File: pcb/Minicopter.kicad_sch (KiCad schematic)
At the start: 0 parts

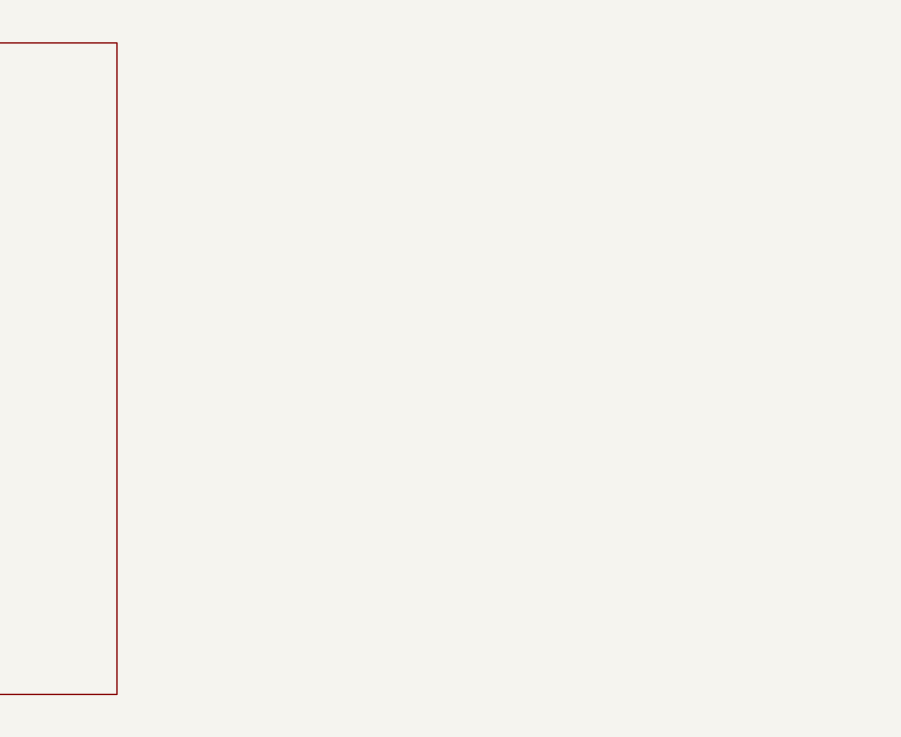
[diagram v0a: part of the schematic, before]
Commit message: battery
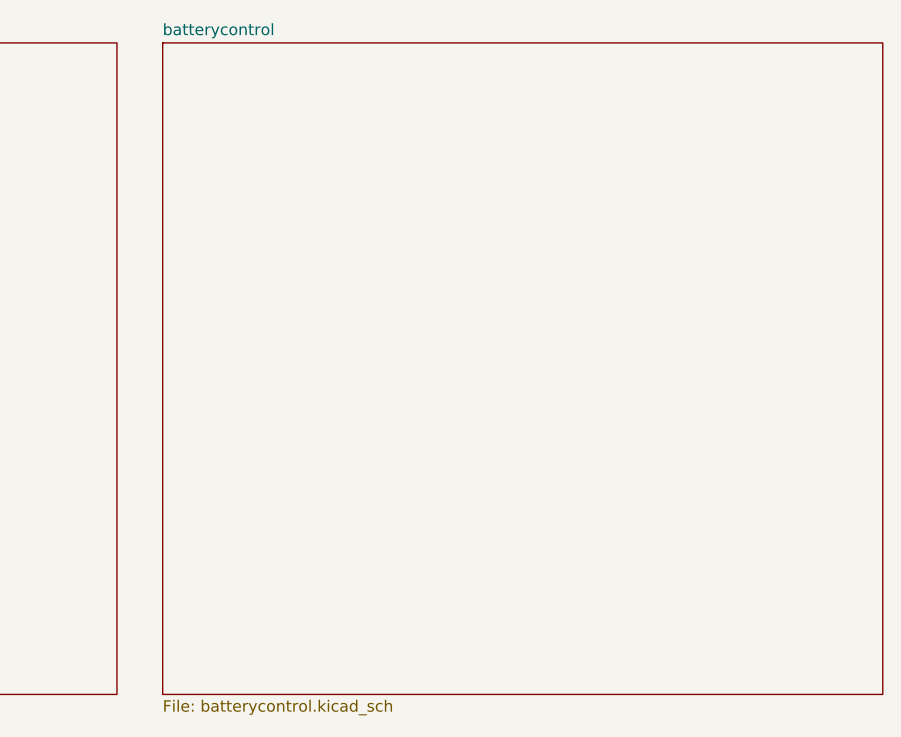
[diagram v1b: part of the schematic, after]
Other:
- added sheet batterycontrol (batterycontrol.kicad_sch)
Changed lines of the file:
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@@
+	)
+	(sheet
+		(at 201.93 17.78)
+		(size 80.01 72.39)
+		(exclude_from_sim no)
+		(in_bom yes)
+		(on_board yes)
+		(dnp no)
+		(fields_autoplaced yes)
+		(stroke
+			(width 0.1524)
+			(type solid)
+		)
+		(fill
+			(color 0 0 0 0.0000)
+		)
+		(property "Sheetname" "batterycontrol"
+			(at 201.93 17.0684 0)
+			(effects
+				(font
+					(size 1.27 1.27)
+				)
+				(justify left bottom)
+			)
+		)
+		(property "Sheetfile" "batterycontrol.kicad_sch"
+			(at 201.93 90.7546 0)
+			(effects
+				(font
+					(size 1.27 1.27)
+				)
+				(justify left top)
+			)
+		)
+		(instances
+			(project "Minicopter"
+				(path "/64f47f0f-737f-4ea8-9b68-9c8ed6450afb"
+					(page "4")
+				)
+			)
+		)
 	)
 	(sheet

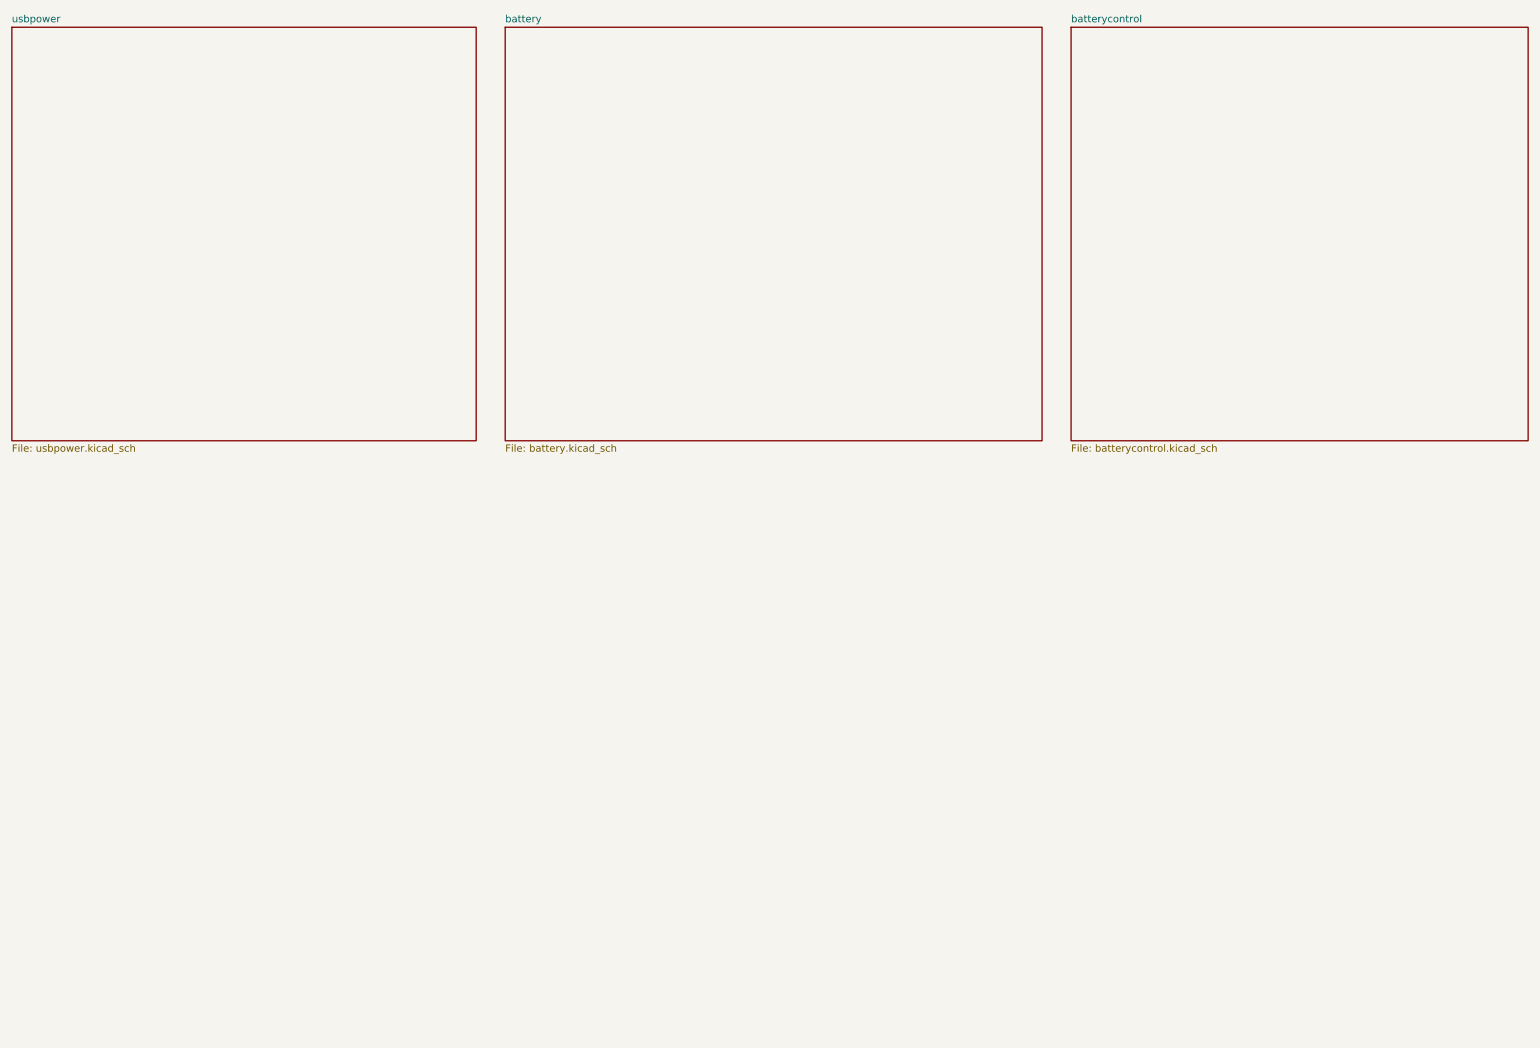
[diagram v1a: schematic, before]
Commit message: with errors
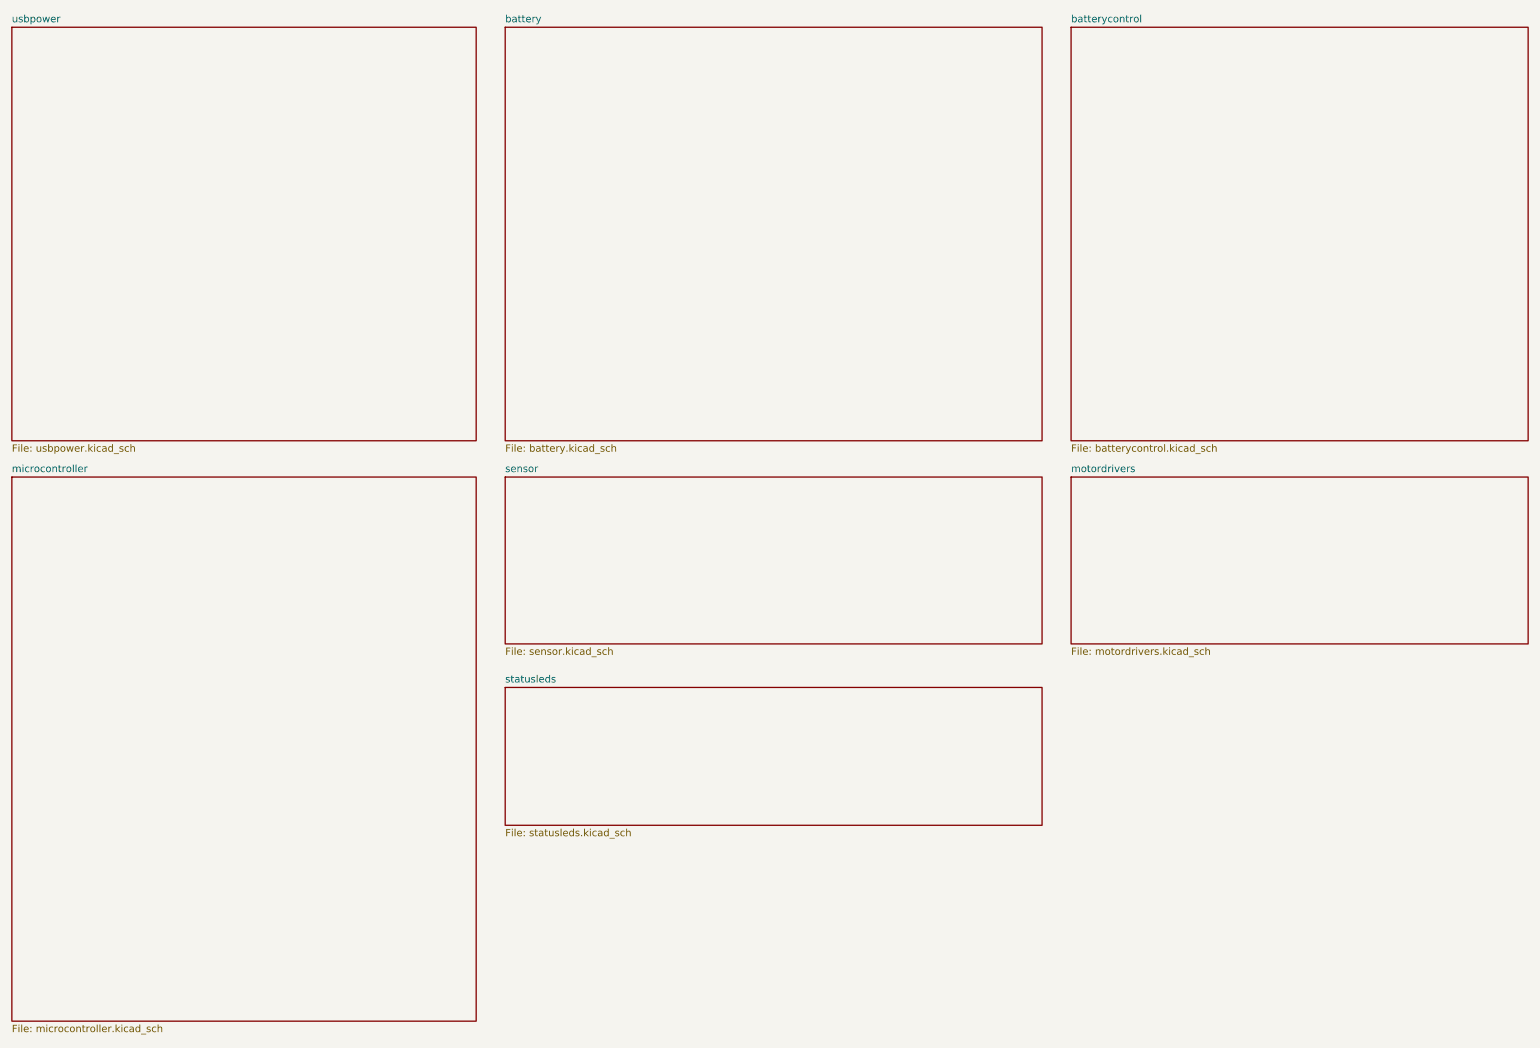
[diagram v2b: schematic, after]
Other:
- added sheet microcontroller (microcontroller.kicad_sch)
- added sheet motordrivers (motordrivers.kicad_sch)
- added sheet sensor (sensor.kicad_sch)
- added sheet statusleds (statusleds.kicad_sch)
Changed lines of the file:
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@@
+	)
+	(sheet
+		(at 16.51 96.52)
+		(size 81.28 95.25)
+		(exclude_from_sim no)
+		(in_bom yes)
+		(on_board yes)
+		(dnp no)
+		(fields_autoplaced yes)
+		(stroke
+			(width 0.1524)
+			(type solid)
+		)
+		(fill
+			(color 0 0 0 0.0000)
+		)
+		(property "Sheetname" "microcontroller"
+			(at 16.51 95.8084 0)
+			(effects
+				(font
+					(size 1.27 1.27)
+				)
+				(justify left bottom)
+			)
+		)
+		(property "Sheetfile" "microcontroller.kicad_sch"
+			(at 16.51 192.3546 0)
+			(effects
+				(font
+					(size 1.27 1.27)
+				)
+				(justify left top)
+			)
+		)
+		(instances
+			(project "Minicopter"
+				(path "/64f47f0f-737f-4ea8-9b68-9c8ed6450afb"
+					(page "5")
+				)
+			)
+		)
 	)
 	(sheet
@@
 				)
 			)
+		)
+	)
+	(sheet
+		(at 102.87 96.52)
+		(size 93.98 29.21)
+		(exclude_from_sim no)
+		(in_bom yes)
+		(on_board yes)
+		(dnp no)
+		(fields_autoplaced yes)
+		(stroke
+			(width 0.1524)
+			(type solid)
+		)
+		(fill
+			(color 0 0 0 0.0000)
+		)
+		(property "Sheetname" "sensor"
+			(at 102.87 95.8084 0)
+			(effects
+				(font
+					(size 1.27 1.27)
+				)
+				(justify left bottom)
+			)
+		)
+		(property "Sheetfile" "sensor.kicad_sch"
+			(at 102.87 126.3146 0)
+			(effects
+				(font
+					(size 1.27 1.27)
+				)
+				(justify left top)
+			)
+		)
+		(instances
+			(project "Minicopter"
+				(path "/64f47f0f-737f-4ea8-9b68-9c8ed6450afb"
+					(page "6")
+				)
+			)
+		)
+	)
+	(sheet
+		(at 201.93 96.52)
+		(size 80.01 29.21)
+		(exclude_from_sim no)
+		(in_bom yes)
+		(on_board yes)
+		(dnp no)
+		(fields_autoplaced yes)
+		(stroke
+			(width 0.1524)
+			(type solid)
+		)
+		(fill
+			(color 0 0 0 0.0000)
+		)
+		(property "Sheetname" "motordrivers"
+			(at 201.93 95.8084 0)
+			(effects
+				(font
+					(size 1.27 1.27)
+				)
+				(justify left bottom)
+			)
+		)
+		(property "Sheetfile" "motordrivers.kicad_sch"
+			(at 201.93 126.3146 0)
+			(effects
+				(font
+					(size 1.27 1.27)
+				)
+				(justify left top)
+			)
+		)
+		(instances
+			(project "Minicopter"
+				(path "/64f47f0f-737f-4ea8-9b68-9c8ed6450afb"
+					(page "7")
+				)
+			)
+		)
+	)
+	(sheet
+		(at 102.87 133.35)
+		(size 93.98 24.13)
+		(exclude_from_sim no)
+		(in_bom yes)
+		(on_board yes)
+		(dnp no)
+		(fields_autoplaced yes)
+		(stroke
+			(width 0.1524)
+			(type solid)
+		)
+		(fill
+			(color 0 0 0 0.0000)
+		)
+		(property "Sheetname" "statusleds"
+			(at 102.87 132.6384 0)
+			(effects
+				(font
+					(size 1.27 1.27)
+				)
+				(justify left bottom)
+			)
+		)
+		(property "Sheetfile" "statusleds.kicad_sch"
+			(at 102.87 158.0646 0)
+			(effects
+				(font
+					(size 1.27 1.27)
+				)
+				(justify left top)
+			)
+		)
+		(instances
+			(project "Minicopter"
+				(path "/64f47f0f-737f-4ea8-9b68-9c8ed6450afb"
+					(page "8")
+				)
+			)

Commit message: finished schematic
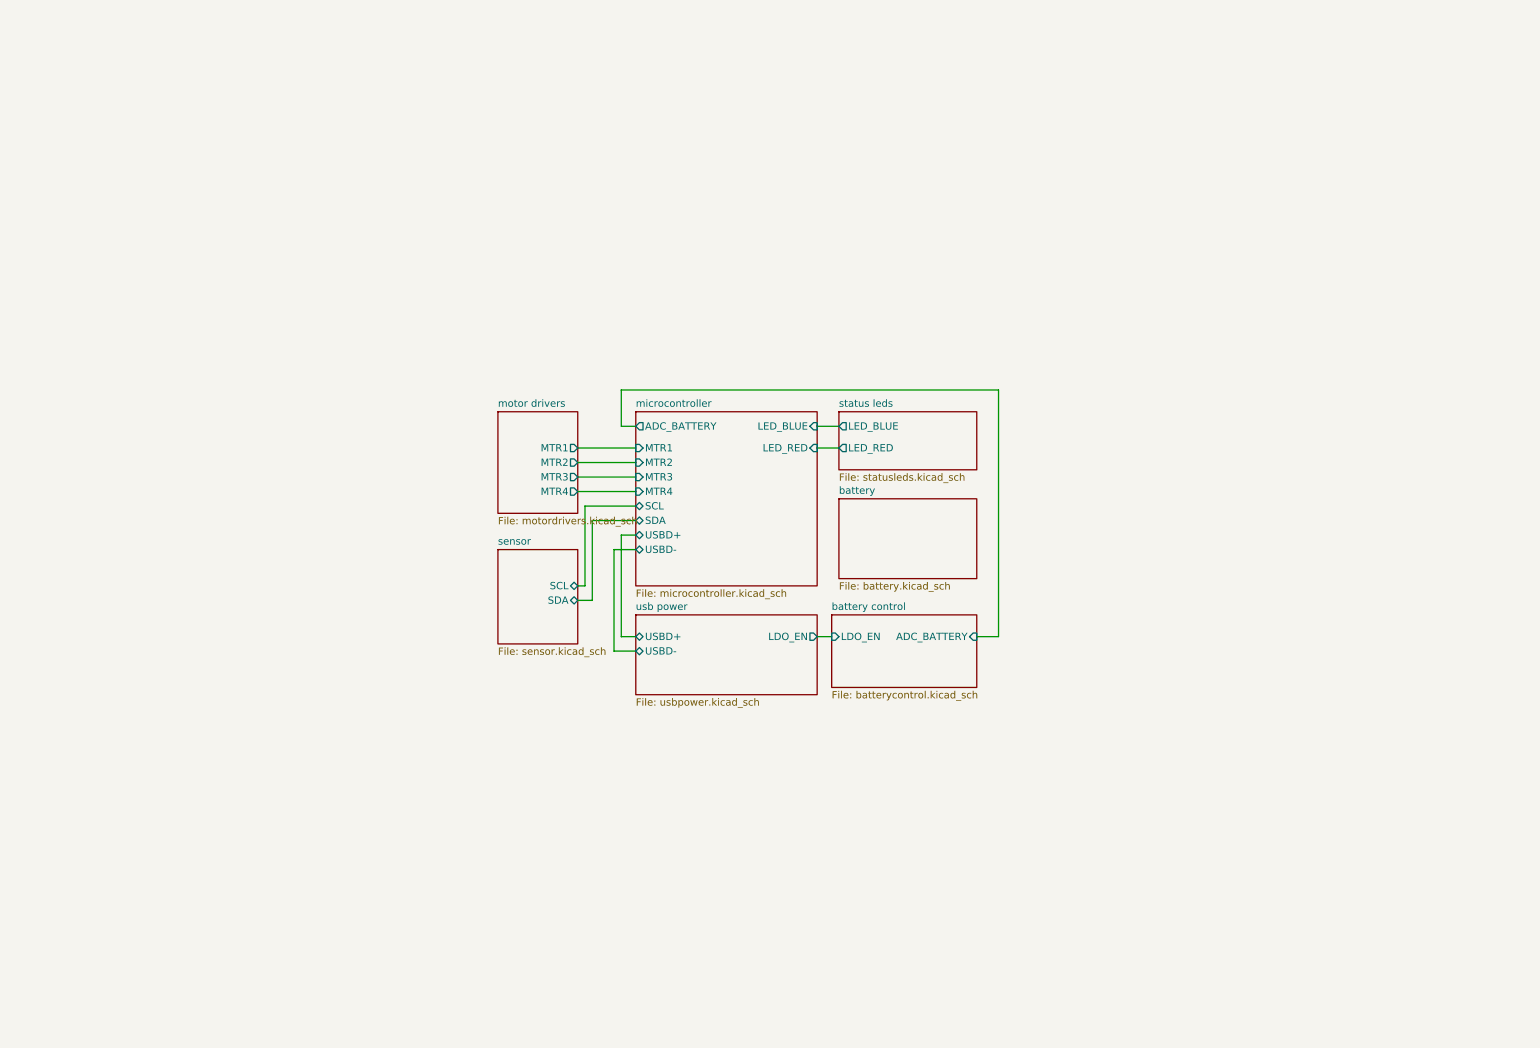
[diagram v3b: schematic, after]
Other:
- removed sheet batterycontrol
- removed sheet motordrivers
- removed sheet statusleds
- removed sheet usbpower
- added sheet battery control (batterycontrol.kicad_sch)
- added sheet motor drivers (motordrivers.kicad_sch)
- added sheet status leds (statusleds.kicad_sch)
- added sheet usb power (usbpower.kicad_sch)
- sheet microcontroller ports: added ADC_BATTERY, LED_BLUE, LED_RED, MTR1, MTR2, MTR3, MTR4, SCL, SDA, USBD+, USBD-; removed none
- sheet sensor ports: added SCL, SDA; removed none
